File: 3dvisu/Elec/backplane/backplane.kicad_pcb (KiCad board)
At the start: 2 copper layers, 99 x 149 mm, 39 parts, among them J1 Jack-DC, J10 Conn_02x10_Counter_Clockwise, J11 Conn_02x10_Counter_Clockwise, J12 Conn_01x01, J13 Conn_01x01, J14 Conn_01x01, J15 Conn_01x01, J2 USB_C_Receptacle, J3 Conn_02x10_Counter_Clockwise, J4 Conn_02x10_Counter_Clockwise, J5 Conn_02x20_Counter_Clockwise, J6 Conn_02x10_Counter_Clockwise, J7 Conn_02x10_Counter_Clockwise, J8 Conn_02x10_Counter_Clockwise, J9 Conn_02x10_Counter_Clockwise, U1 L7805, U2 FT230XS, U3 STM32H753ZITx, U4 TJA1021T, U5 TJA1021T, Y1 Crystal

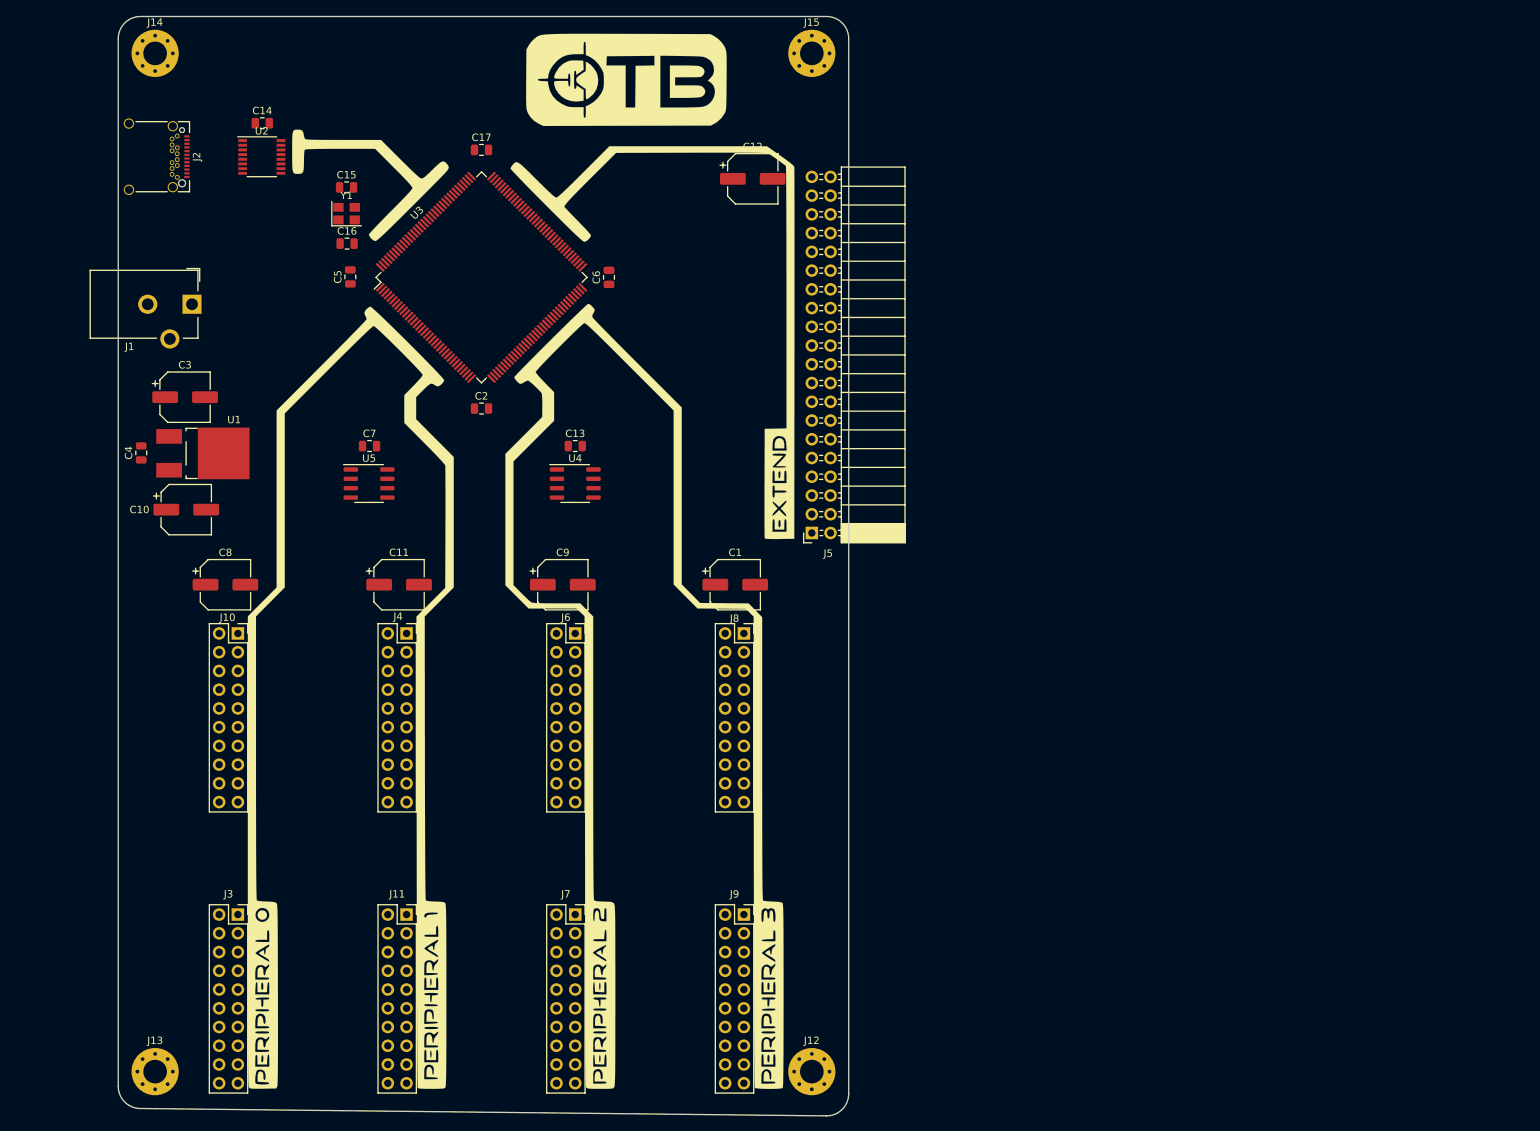
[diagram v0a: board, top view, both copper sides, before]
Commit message: render made
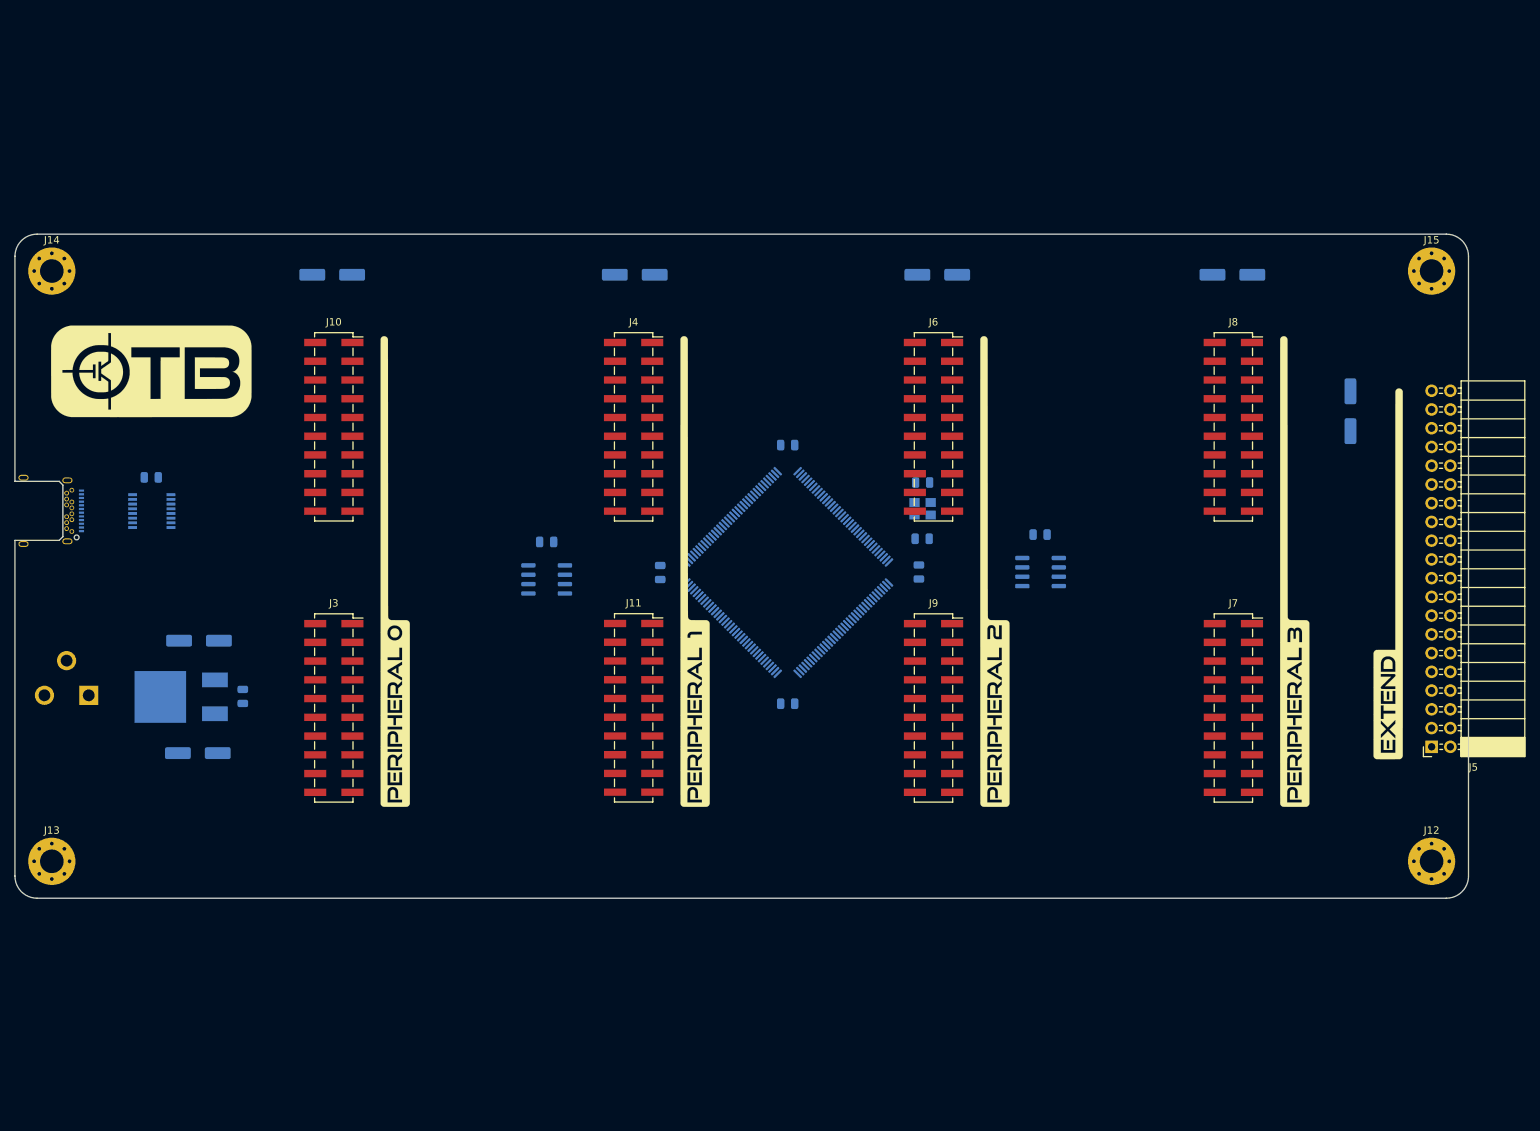
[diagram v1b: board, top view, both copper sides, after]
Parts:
- removed the G*** at (115.6, 92.8)
- added G***: LOGO, MyLibKicad:serigback, F.Cu at (143.5, 93.5)
- C1, C10, C11, C12, C13, C14, C15, C16, C17, C2, C3, C4, C5, C6, C7, C8, C9, J1, U1, U2, U3, U4, U5, Y1: moved to B.Cu
- J10, J11, J3, J4, J6, J7, J8, J9: footprint Connector_PinSocket_2.54mm:PinSocket_2x10_P2.54mm_Vertical -> Connector_PinSocket_2.54mm:PinSocket_2x10_P2.54mm_Vertical_SMD
- J2: footprint Connector_USB:USB_C_Receptacle_Amphenol_12401548E4-2A_CircularHoles -> Connector_USB:USB_C_Receptacle_Amphenol_12401548E4-2A; moved to B.Cu
- moved C8 142.8 mm to (212.0, 54.0)
- moved J7 93.5 mm to (212.1, 112.7)
- moved U5 91.8 mm to (186.0, 94.3), turned to 180 degrees
- moved C7 91.7 mm to (185.9, 89.2), turned to 180 degrees
- moved J15 89.0 mm to (239.0, 53.5)
- moved J5 88.9 mm to (239.0, 118.0)
- moved J12 88.7 mm to (239.0, 133.5)
- moved C15 87.7 mm to (170.0, 82.2), turned to 180 degrees
- moved Y1 87.7 mm to (170.0, 85.7), turned to 180 degrees
- moved C16 87.6 mm to (170.0, 89.8), turned to 180 degrees
- moved C12 86.9 mm to (228.0, 72.5), turned to 270 degrees
- moved C5 86.8 mm to (169.5, 94.3)
- moved J8 72.0 mm to (212.1, 74.6)
- moved U3 57.6 mm to (151.7, 94.4), turned to 135 degrees
- moved C17 57.6 mm to (151.7, 77.1), turned to 180 degrees
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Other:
- board size 99 x 149 mm -> 197 x 90 mm
